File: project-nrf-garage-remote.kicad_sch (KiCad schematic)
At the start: 9 parts, among them J1 Screw_Terminal_01x02, J2 Screw_Terminal_01x04, Q1 BSS138W, Q2 BSS138W

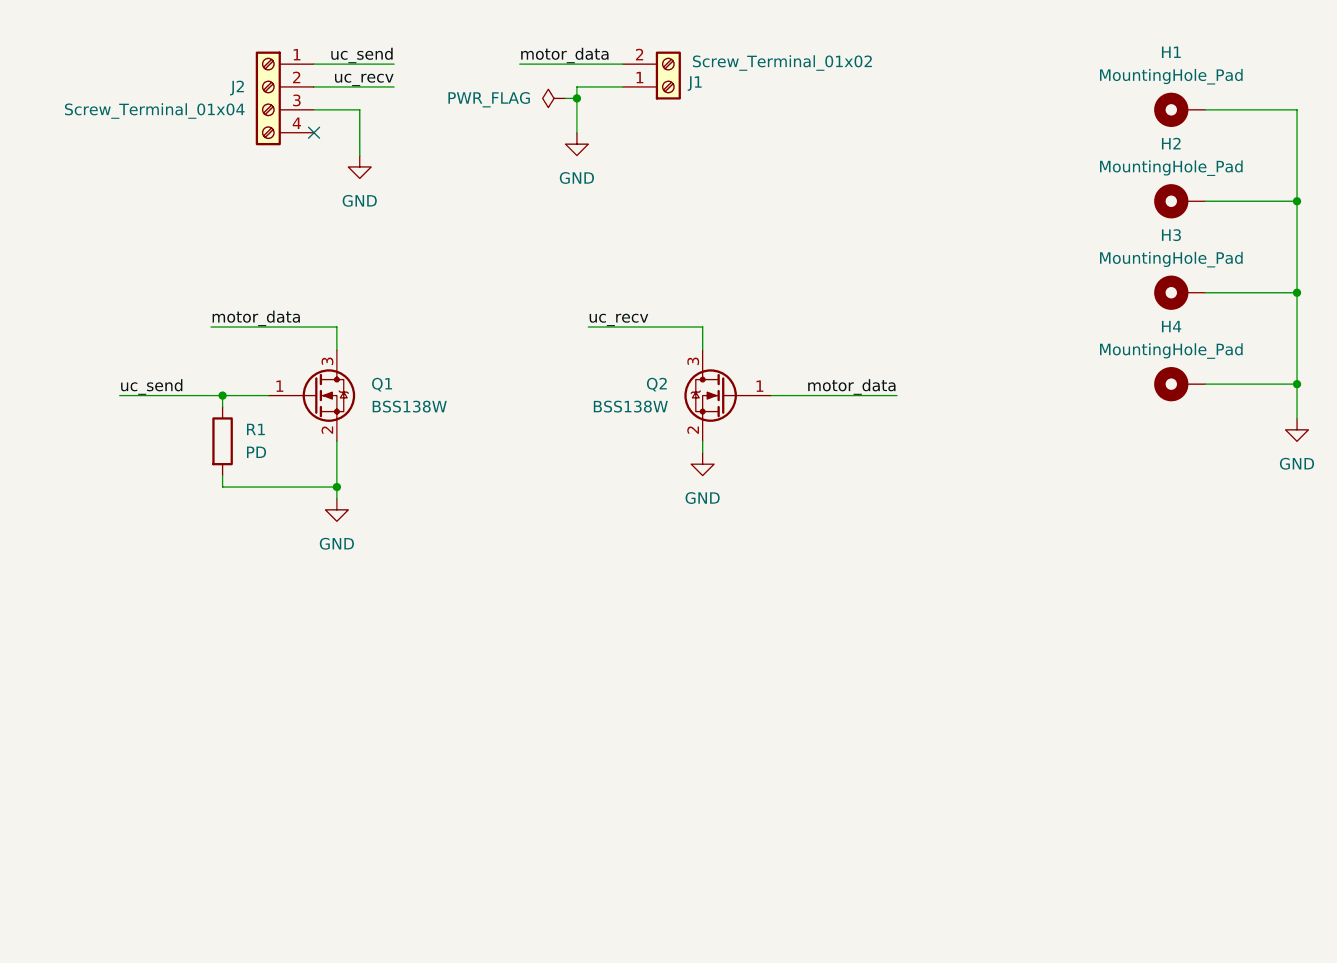
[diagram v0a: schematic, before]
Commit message: Update schematic
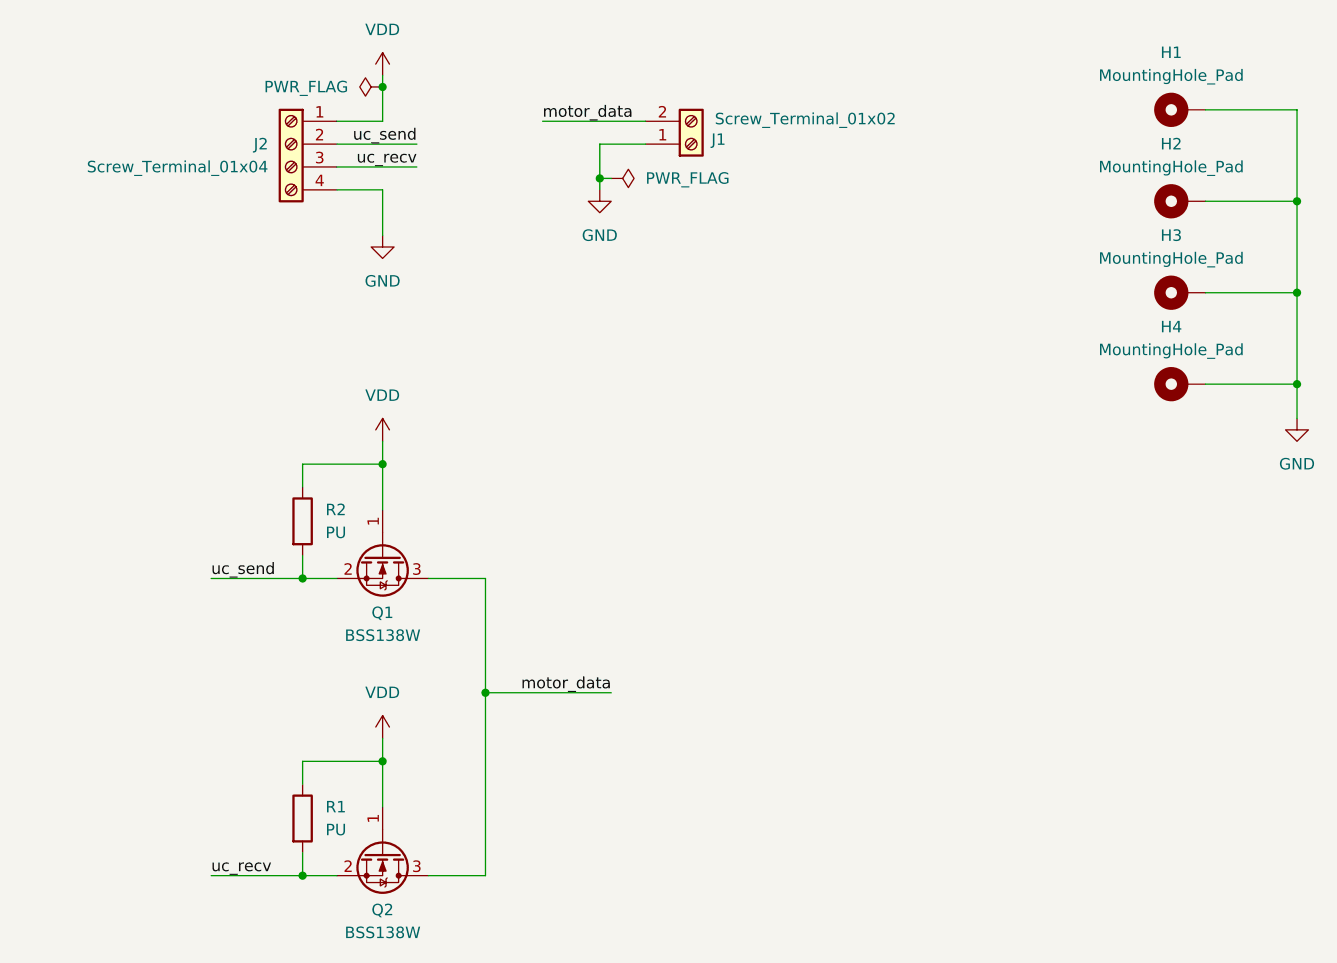
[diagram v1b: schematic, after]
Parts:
- added R2: PU, Resistor_SMD:R_0603_1608Metric, symbol Device:R
- R1: value PD -> PU
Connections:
- net GND: now also J2.4 (Pin_4); no longer J2.3 (Pin_3), Q1.2 (S), Q2.2 (S), R1.2
- net motor_data: now also Q2.3 (D); no longer Q2.1 (G)
- net uc_recv: now also J2.3 (Pin_3), Q2.2 (S), R1.2; no longer J2.2 (Pin_2), Q2.3 (D)
- net uc_send: now also J2.2 (Pin_2), Q1.2 (S), R2.2; no longer J2.1 (Pin_1), Q1.1 (G), R1.1
- new net VDD: J2.1 (Pin_1), Q1.1 (G), Q2.1 (G), R1.1, R2.1
- no-connect marks 1 -> 0
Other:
- moved on the sheet: J1, J2, Q1, Q2, R1
